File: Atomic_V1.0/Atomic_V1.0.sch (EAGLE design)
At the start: 14 parts, among them U4 TLE9250VSJ, X1 S4P-VH

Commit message: made PDF
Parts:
- C1: value 22µF -> 47uF
- D2: value S1ML -> SS12L R3
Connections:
- net CAN_N renamed CAN_L
- net CAN_P renamed CAN_H

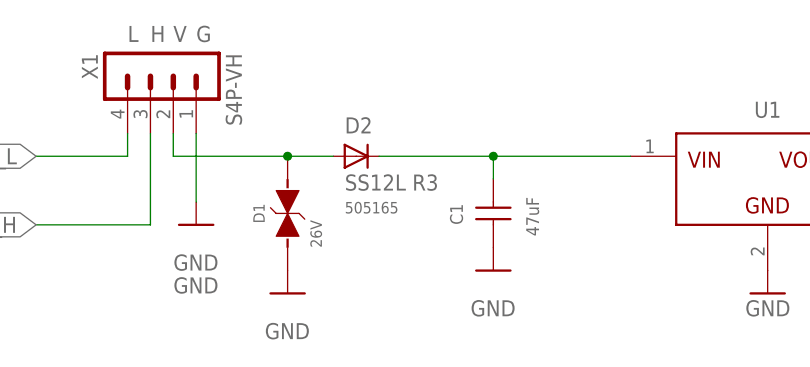
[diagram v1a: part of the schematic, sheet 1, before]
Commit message: DCDC Version
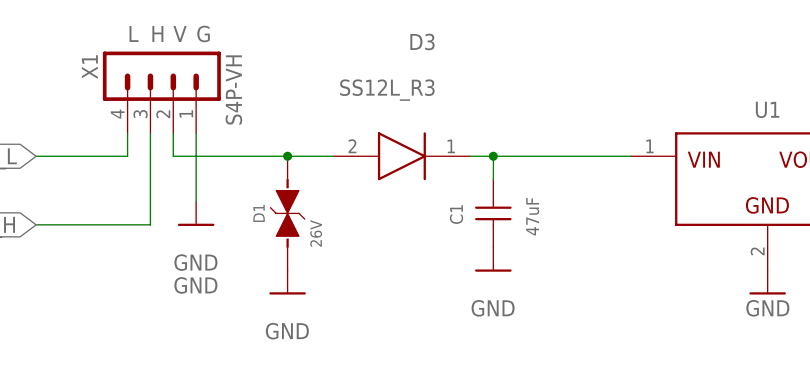
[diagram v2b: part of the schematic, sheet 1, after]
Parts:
- removed D2: SS12L R3, fliegl-elektronik:S1ML
- added D3: SS12L_R3, SS12L_R3:SS12L_R3
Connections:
- net +12V: now also D3.A; no longer D2.A
- net N$1: now also D3.K; no longer D2.C
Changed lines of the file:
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@@
 <part name="P+3" library="supply1" deviceset="+5V" device=""/>
 <part name="D1" library="Wurth_EMC Components_WE-TVSP" library_urn="urn:adsk.eagle:library:14283044" deviceset="WE-TVSP_DO-214AC_400W_BI" device="" package3d_urn="urn:adsk.eagle:package:12146531/2" technology="_824501261" value="26V"/>
-<part name="D2" library="fliegl-elektronik" deviceset="S1ML" device="" value="SS12L R3"/>
 <part name="GND4" library="supply1" deviceset="GND" device=""/>
 <part name="C1" library="Wurth_Capacitors_WCAP-CSGP" library_urn="urn:adsk.eagle:library:18488985" deviceset="WCAP-CSGP_1210_H2.5" device="_25V(DC)" package3d_urn="urn:adsk.eagle:package:18489097/2" technology="_885012109014" value="47uF"/>
 <part name="GND6" library="supply1" deviceset="GND" device=""/>
+<part name="D3" library="SS12L_R3" deviceset="SS12L_R3" device=""/>
 </parts>
 <sheets>
@@
 <attribute name="VALUE" x="-11.43" y="116.84" size="1.27" layer="95" rot="R90"/>
 </instance>
-<instance part="D2" gate="G$1" x="-7.62" y="127" smashed="yes">
-<attribute name="NAME" x="-8.89" y="129.54" size="1.778" layer="95"/>
-<attribute name="VALUE" x="-8.89" y="123.19" size="1.778" layer="96"/>
-<attribute name="ARTIKEL_NR" x="-8.89" y="120.65" size="1.27" layer="96"/>
-</instance>
 <instance part="GND4" gate="1" x="-15.24" y="111.76" smashed="yes">
 <attribute name="VALUE" x="-17.78" y="106.68" size="1.778" layer="96"/>
@@
 <instance part="GND6" gate="1" x="7.62" y="114.3" smashed="yes">
 <attribute name="VALUE" x="5.08" y="109.22" size="1.778" layer="96"/>
+</instance>
+<instance part="D3" gate="G$1" x="5.08" y="127" smashed="yes" rot="R180">
+<attribute name="NAME" x="1.27" y="139.7" size="1.778" layer="95" rot="R180" align="center-left"/>
+<attribute name="VALUE" x="1.27" y="134.62" size="1.778" layer="96" rot="R180" align="center-left"/>
 </instance>
 </instances>
@@
 <pinref part="X1" gate="G$1" pin="2"/>
 <wire x1="-27.94" y1="129.54" x2="-27.94" y2="127" width="0.1524" layer="91"/>
-<pinref part="D2" gate="G$1" pin="A"/>
+<pinref part="D1" gate="G$1" pin="2"/>
 <wire x1="-10.16" y1="127" x2="-15.24" y2="127" width="0.1524" layer="91"/>
-<pinref part="D1" gate="G$1" pin="2"/>
 <wire x1="-15.24" y1="127" x2="-27.94" y2="127" width="0.1524" layer="91"/>
 <junction x="-15.24" y="127"/>
+<pinref part="D3" gate="G$1" pin="A"/>
 </segment>
 </net>
@@
 <segment>
 <pinref part="U1" gate="G$1" pin="VIN"/>
-<pinref part="D2" gate="G$1" pin="C"/>
-<wire x1="-5.08" y1="127" x2="7.62" y2="127" width="0.1524" layer="91"/>
 <pinref part="C1" gate="G$1" pin="2"/>
+<wire x1="5.08" y1="127" x2="7.62" y2="127" width="0.1524" layer="91"/>
 <wire x1="7.62" y1="127" x2="22.86" y2="127" width="0.1524" layer="91"/>
 <wire x1="7.62" y1="124.46" x2="7.62" y2="127" width="0.1524" layer="91"/>
 <junction x="7.62" y="127"/>
+<pinref part="D3" gate="G$1" pin="K"/>
 </segment>
 </net>
